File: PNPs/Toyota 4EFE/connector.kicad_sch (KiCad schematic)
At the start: 9 parts, among them J4 Conn_02x20_Counter_Clockwise, J9 4E-FE OEM

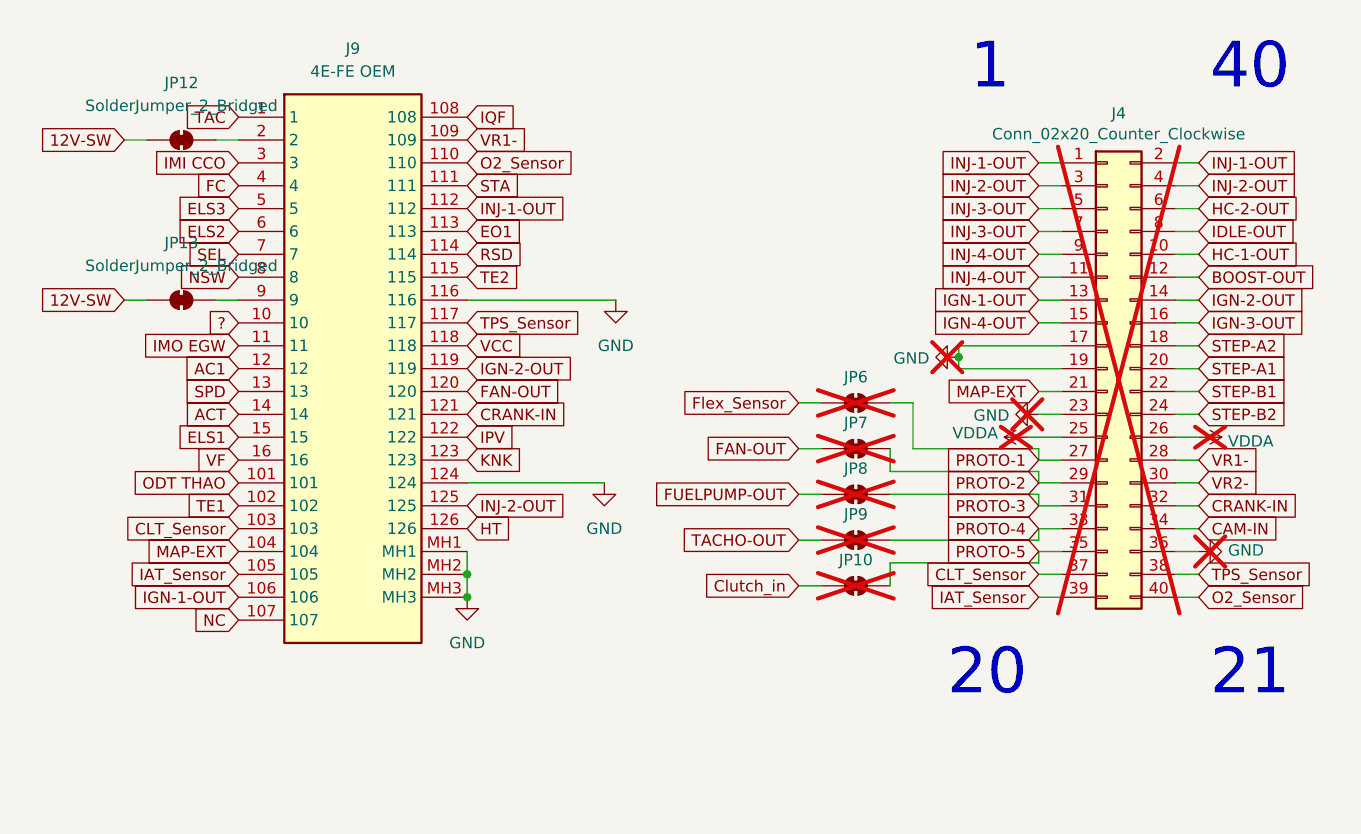
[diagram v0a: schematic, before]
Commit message: Board layout done
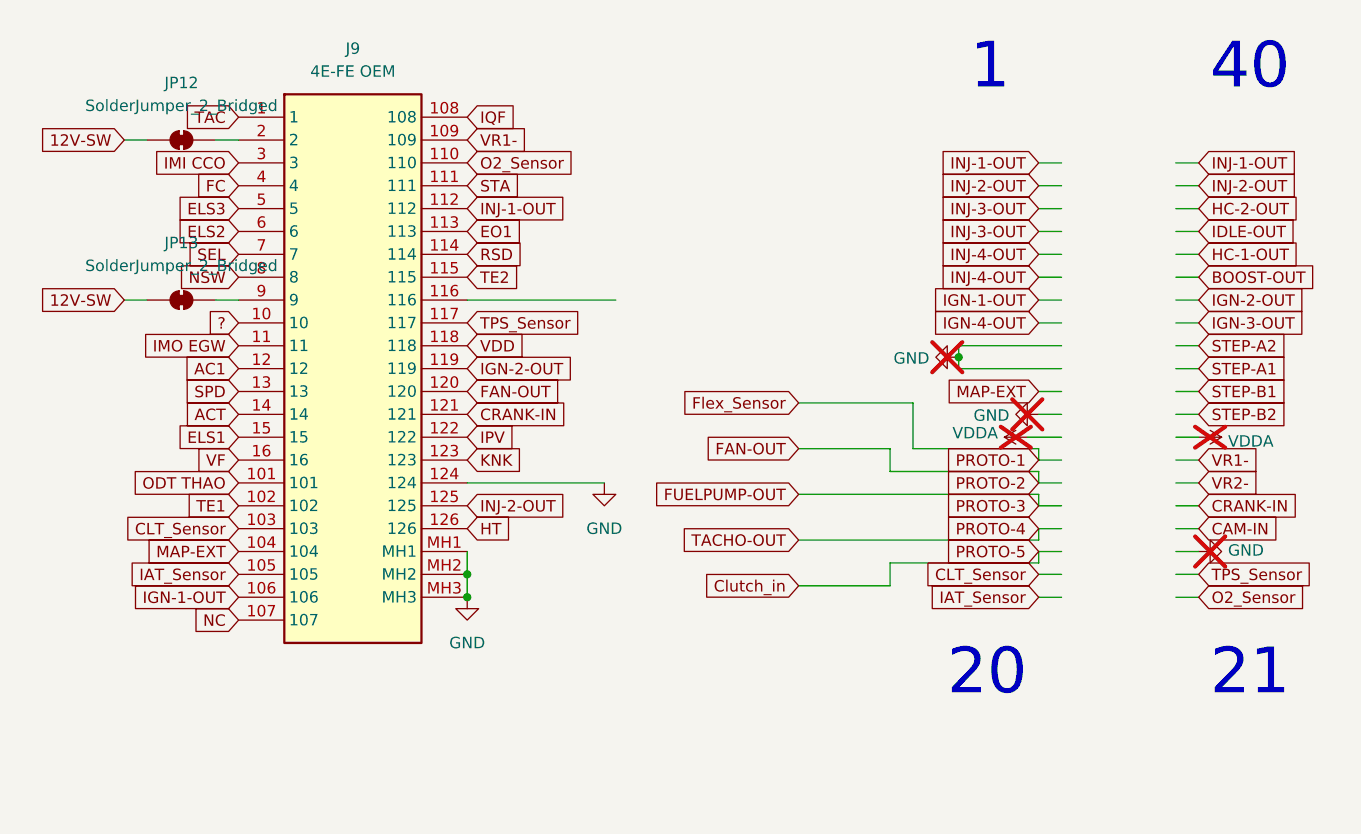
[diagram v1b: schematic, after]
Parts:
- removed J4: Conn_02x20_Counter_Clockwise, Connector_IDC:IDC-Header_2x20_P2.54mm_Vertical, symbol Connector_Generic:Conn_02x20_Odd_Even
- removed JP10, JP6, JP7, JP8, JP9: SolderJumper_2_Bridged, Jumper:SolderJumper-2_P1.3mm_Bridged_Pad1.0x1.5mm, symbol Jumper:SolderJumper_2_Bridged
- J9: footprint 175446-6:1754466 -> (none)
- JP12, JP13: footprint Jumper:SolderJumper-2_P1.3mm_Bridged_Pad1.0x1.5mm -> (none)
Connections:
- net GND: no longer J9.116
- net VCC renamed VDD

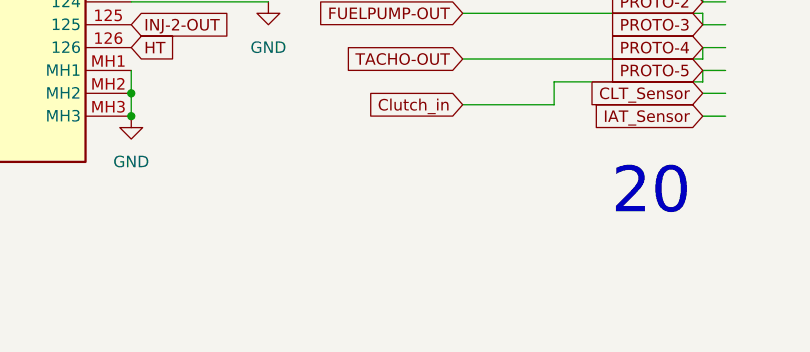
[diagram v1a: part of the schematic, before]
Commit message: Added annotations etc.
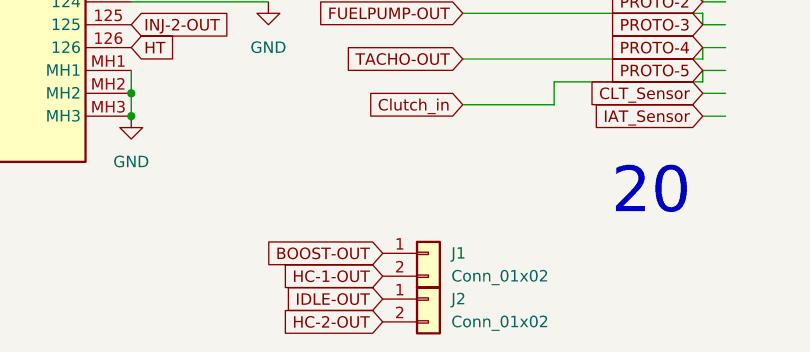
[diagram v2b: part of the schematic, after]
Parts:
- added J1, J2: Conn_01x02, Connector_PinHeader_2.54mm:PinHeader_1x02_P2.54mm_Vertical, symbol Connector_Generic:Conn_01x02
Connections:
- net BOOST-OUT: now also J1.1 (Pin_1)
- net HC-1-OUT: now also J1.2 (Pin_2)
- net HC-2-OUT: now also J2.2 (Pin_2)
- net IDLE-OUT: now also J2.1 (Pin_1)
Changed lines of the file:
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@@
+		)
+	)
+	(global_label "HC-1-OUT"
+		(shape input)
+		(at 111.76 139.7 180)
+		(effects
+			(font
+				(size 1.27 1.27)
+			)
+			(justify right)
+		)
+		(property "Intersheetrefs" "${INTERSHEET_REFS}"
+			(at 111.76 139.7 0)
+			(effects
+				(font
+					(size 1.27 1.27)
+				)
+				(hide yes)
+			)
 		)
 	)
@@
 		)
 	)
+	(global_label "HC-2-OUT"
+		(shape input)
+		(at 111.76 144.78 180)
+		(effects
+			(font
+				(size 1.27 1.27)
+			)
+			(justify right)
+		)
+		(property "Intersheetrefs" "${INTERSHEET_REFS}"
+			(at 111.76 144.78 0)
+			(effects
+				(font
+					(size 1.27 1.27)
+				)
+				(hide yes)
+			)
+		)
+	)
 	(global_label "Flex_Sensor"
 		(shape input)
@@
 		)
 	)
+	(global_label "IDLE-OUT"
+		(shape input)
+		(at 111.76 142.24 180)
+		(effects
+			(font
+				(size 1.27 1.27)
+			)
+			(justify right)
+		)
+		(property "Intersheetrefs" "${INTERSHEET_REFS}"
+			(at 111.76 142.24 0)
+			(effects
+				(font
+					(size 1.27 1.27)
+				)
+				(hide yes)
+			)
+		)
+	)
 	(global_label "FUELPUMP-OUT"
 		(shape input)
@@
 		(property "Intersheetrefs" "${INTERSHEET_REFS}"
 			(at 58.42 119.38 0)
+			(effects
+				(font
+					(size 1.27 1.27)
+				)
+				(hide yes)
+			)
+		)
+	)
+	(global_label "BOOST-OUT"
+		(shape input)
+		(at 111.76 137.16 180)
+		(effects
+			(font
+				(size 1.27 1.27)
+			)
+			(justify right)
+		)
+		(property "Intersheetrefs" "${INTERSHEET_REFS}"
+			(at 111.76 137.16 0)
 			(effects
 				(font
@@
 					(unit 1)
 				)
+			)
+		)
+	)
+	(symbol
+		(lib_id "Connector_Generic:Conn_01x02")
+		(at 116.84 137.16 0)
+		(unit 1)
+		(exclude_from_sim no)
+		(in_bom yes)
+		(on_board yes)
+		(dnp no)
+		(fields_autoplaced yes)
+		(property "Reference" "J1"
+			(at 119.38 137.1599 0)
+			(effects
+				(font
+					(size 1.27 1.27)
+				)
+				(justify left)
+			)
+		)
+		(property "Value" "Conn_01x02"
+			(at 119.38 139.6999 0)
+			(effects
+				(font
+					(size 1.27 1.27)
+				)
+				(justify left)
+			)
+		)
+		(property "Footprint" "Connector_PinHeader_2.54mm:PinHeader_1x02_P2.54mm_Vertical"
+			(at 116.84 137.16 0)
+			(effects
+				(font
+					(size 1.27 1.27)
+				)
+				(hide yes)
+			)
+		)
+		(property "Datasheet" "~"
+			(at 116.84 137.16 0)
+			(effects
+				(font
+					(size 1.27 1.27)
+				)
+				(hide yes)
+			)
+		)
+		(property "Description" "Generic connector, single row, 01x02, script generated (kicad-library-utils/schlib/autogen/connector/)"
+			(at 116.84 137.16 0)
+			(effects
+				(font
+					(size 1.27 1.27)
+				)
+				(hide yes)
+			)
+		)
+		(pin "2"
+		)
+		(pin "1"
+		)
+		(instances
+			(project ""
+				(path "/04f7226c-d840-4f7e-960b-f287626b813e/00000000-0000-0000-0000-00005cd19033"
+					(reference "J1")
+					(unit 1)
+				)
+			)
+		)
+	)
+	(symbol
+		(lib_id "Connector_Generic:Conn_01x02")
+		(at 116.84 142.24 0)
+		(unit 1)
+		(exclude_from_sim no)
+		(in_bom yes)
+		(on_board yes)
+		(dnp no)
+		(fields_autoplaced yes)
+		(property "Reference" "J2"
+			(at 119.38 142.2399 0)
+			(effects
+				(font
+					(size 1.27 1.27)
+				)
+				(justify left)
+			)
+		)
+		(property "Value" "Conn_01x02"
+			(at 119.38 144.7799 0)
+			(effects
+				(font
+					(size 1.27 1.27)
+				)
+				(justify left)
+			)
+		)
+		(property "Footprint" "Connector_PinHeader_2.54mm:PinHeader_1x02_P2.54mm_Vertical"
+			(at 116.84 142.24 0)
+			(effects
+				(font
+					(size 1.27 1.27)
+				)
+				(hide yes)
+			)
+		)
+		(property "Datasheet" "~"
+			(at 116.84 142.24 0)
+			(effects
+				(font
+					(size 1.27 1.27)
+				)
+				(hide yes)
+			)
+		)
+		(property "Description" "Generic connector, single row, 01x02, script generated (kicad-library-utils/schlib/autogen/connector/)"
+			(at 116.84 142.24 0)
+			(effects
+				(font
+					(size 1.27 1.27)
+				)
+				(hide yes)
+			)
+		)
+		(pin "2"
+		)
+		(pin "1"
+		)
+		(instances
+			(project "toyota 4efe"
+				(path "/04f7226c-d840-4f7e-960b-f287626b813e/00000000-0000-0000-0000-00005cd19033"
+					(reference "J2")
+					(unit 1)
+				)
